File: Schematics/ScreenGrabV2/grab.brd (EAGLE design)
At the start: 48 x 60.4 mm, 48 parts

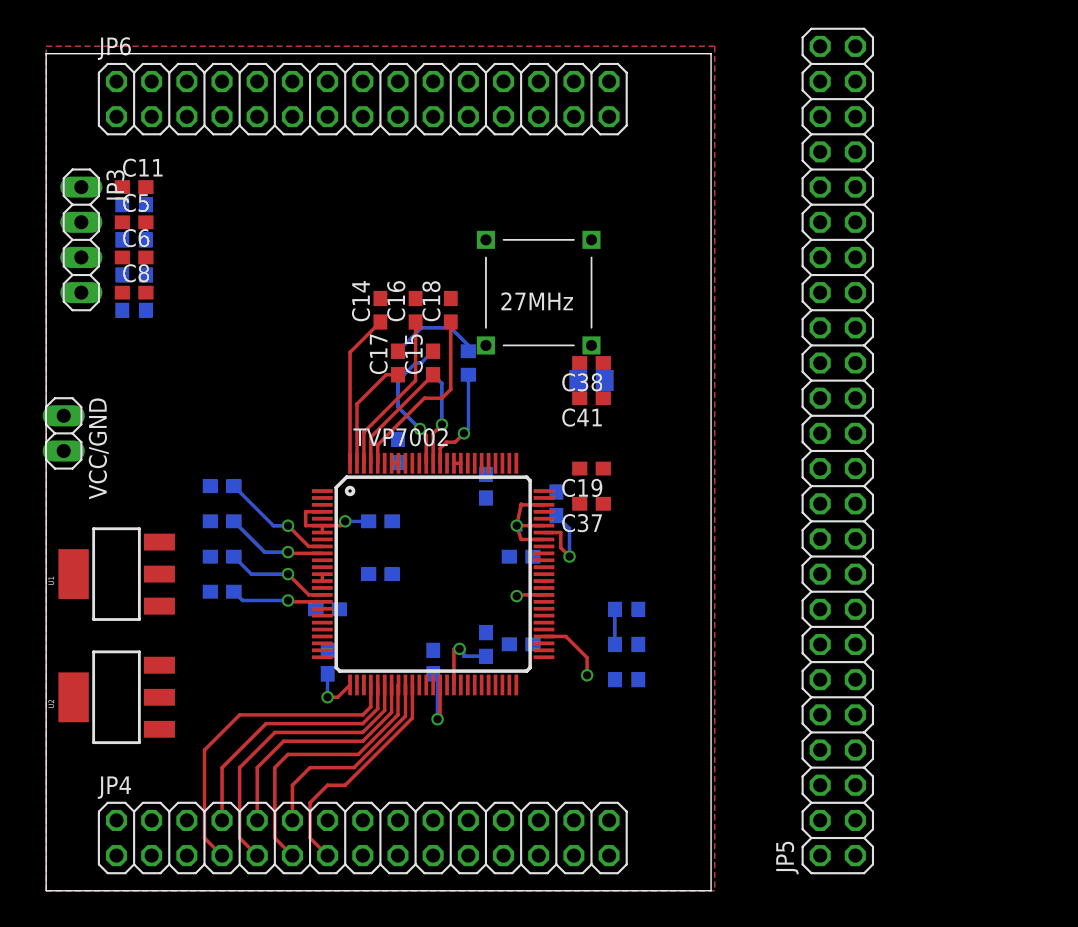
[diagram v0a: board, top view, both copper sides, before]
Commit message: Schematic routed
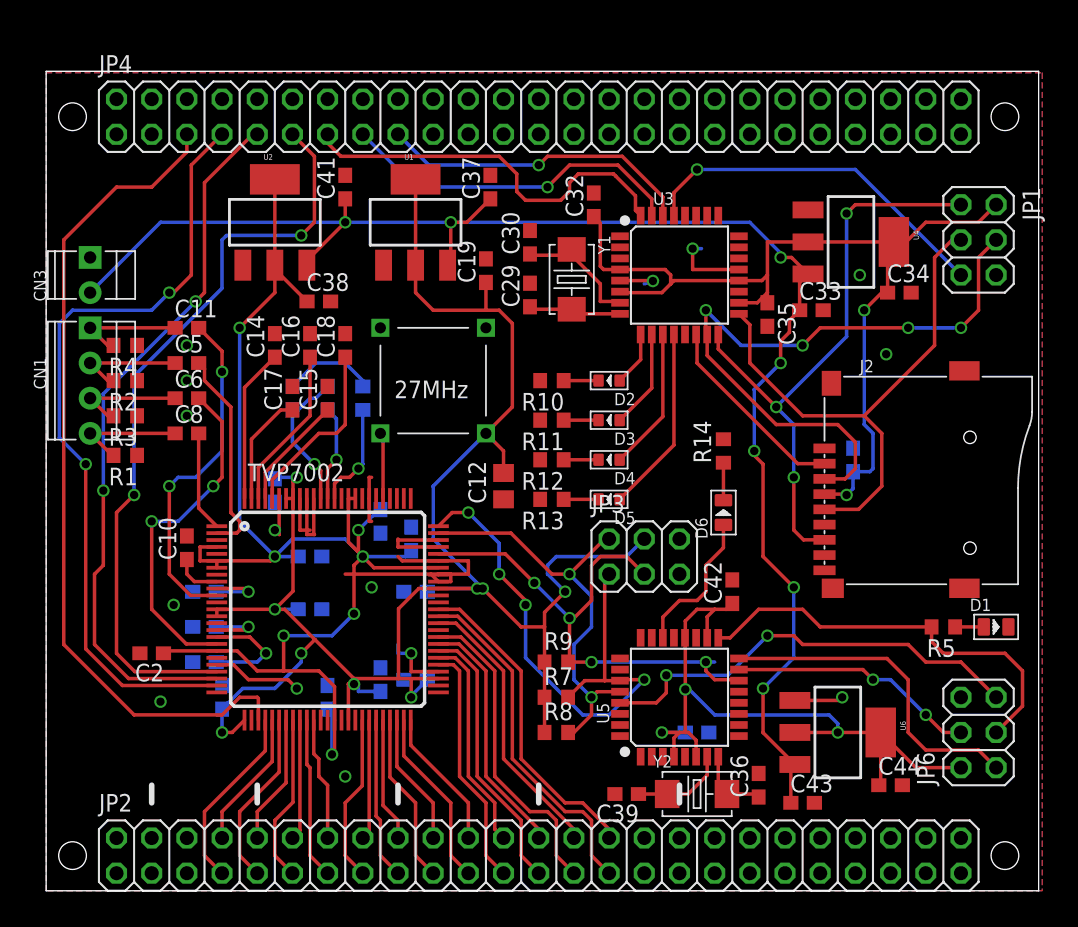
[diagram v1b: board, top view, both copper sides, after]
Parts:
- removed JP5: (no value), pinhead:2X24
- removed VCC/GND: (no value), pinhead:1X02
- added C29, C30, C31, C32, C33, C34, C35, C36, C39, C42, C43, C44, C45: (no value), resistor:C0603
- added CN1: 4p-2.54-h8.5, Seeed-OPL-Connector:H4-2.54-8.52X6.3MM
- added CN3: 2p-2.54-h8.5, Seeed-OPL-Connector:H2-2.54-3.44X6.3MM
- added D1, D6: CLEAR-BLUE-0805, Seeed-OPL-Diode:LED-0805
- added D2, D3, D4, D5: BLUE-0603, Seeed-OPL-Diode:LED-0603
- added J2: MICROSD-9P, Seeed-OPL-Connector:MICRO-SD9+4P-SMD-16.1X14.5X1.85MM
- added JP1: (no value), pinhead:2X03
- added JP2: (no value), pinhead:2X25
- added R10, R11, R12, R13, R14, R5: (no value), resistor:R0603
- added U3, U5: ATMEGA328P-AU-TQFP32, Seeed-OPL-ic:TQFP32-0.8-7X7MM
- added U4, U6: (no value), SparkFun-PowerIC:SOT223
- added Y1, Y2: 16MHZ, Seeed-OPL-crystal-osctllator:X2-SMD-5.0X3.2X1.3MM
- JP3: device pinhead:1X04 -> pinhead:2X03
- JP4: device pinhead:2X15 -> pinhead:2X25
- JP6: device pinhead:2X15 -> pinhead:2X03
- moved JP6 63.8 mm to (67.3, 11.4), turned to 90 degrees
- moved JP4 53.6 mm to (35.6, 55.9)
- moved JP3 46.6 mm to (43.2, 24.1), turned to 0 degrees
- moved U2 36.1 mm to (16.5, 48.3), turned to 0 degrees
- moved U1 33.3 mm to (26.7, 48.3), turned to 0 degrees
- moved C37 24.0 mm to (32.1, 50.8), turned to 90 degrees
- moved C41 23.4 mm to (21.6, 50.8), turned to 90 degrees
- moved C38 20.2 mm to (19.7, 42.5), turned to 0 degrees
- moved C19 16.2 mm to (31.8, 44.8), turned to 90 degrees
- moved C2 13.1 mm to (7.62, 17.1), flipped to the top, turned to 180 degrees
- moved C11 10.9 mm to (10.2, 40.6)
- moved C5 10.9 mm to (10.2, 38.1)
- moved C6 10.9 mm to (10.2, 35.6)
- moved C8 10.9 mm to (10.2, 33.0)
- moved C26 10.8 mm to (26.4, 25.4)
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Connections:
- new net C_MISO: JP6.1, U5.16
- new net C_MOSI: JP6.4, U5.15
- new net C_RST: JP6.5, U5.29
- new net C_SCK: JP6.3, R5.2, U5.17
- new net C_VCC: C42.1, C44.1, C45.1, JP6.2, U5.18, U5.20, U5.4, U5.6, U6.2, U6.4
- new net N$10: C30.1, U3.7, Y1.1
- new net N$11: C29.1, U3.8, Y1.2
- new net N$12: D2.-, R10.1
- new net N$13: D3.-, R11.1
- new net N$14: D4.-, R12.1
- new net N$15: D5.-, R13.1
- new net N$16: D6.+, U5.22
- new net N$17: D6.-, R14.1
- new net N$2: J2.2, U3.14
- new net N$3: D2.+, U3.9
- new net N$4: C39.1, U5.7, Y2.1
- new net N$5: C36.1, U5.8, Y2.2
- new net N$6: D3.+, U3.10
- new net N$7: D4.+, U3.11
- new net N$8: D1.+, R5.1
- new net N$9: D5.+, U3.12
- new net UNUSED1: JP4.17, U3.30
- new net UNUSED2: JP4.15, U3.31
- new net UNUSED3: JP4.13, U3.32
- new net W_MISO: J2.7, JP1.1, U3.16
- new net W_MOSI: J2.3, JP1.4, U3.15
- new net W_RST: JP1.5, U3.29
- new net W_SCK: J2.5, JP1.3, U3.17
- new net W_VCC: C31.1, C32.1, C34.1, C35.1, J2.4, JP1.2, U3.18, U3.20, U3.4, U3.6, U4.2, U4.4
- net +3.3V: now also JP3.4
- net +5V: now also C33.1, C43.1, CN3.2, U4.3, U6.3; no longer VCC/GND.2
- net B0: now also JP2.14; no longer JP4.14
- net B1: now also JP2.13; no longer JP4.13
- net B2: now also JP2.12; no longer JP4.12
- net B3: now also JP2.11; no longer JP4.11
- net B4: now also JP2.10; no longer JP4.10
- net B5: now also JP2.9; no longer JP4.9
- net B6: now also JP2.8; no longer JP4.8
- net B7: now also JP2.7; no longer JP4.7
- net BIN: now also CN1.3; no longer JP3.3
- net CSYNCIN: now also CN1.4; no longer JP3.4
- net FIDOUT: now also JP4.11; no longer JP6.14
- net G0: now also JP2.22; no longer JP4.22
- net G1: now also JP2.21; no longer JP4.21
- net G2: now also JP2.20; no longer JP4.20
- net G3: now also JP2.19; no longer JP4.19
- net G4: now also JP2.18; no longer JP4.18
- net G5: now also JP2.17; no longer JP4.17
- net G6: now also JP2.16; no longer JP4.16
- net G7: now also JP2.15; no longer JP4.15
- net GIN: now also CN1.2; no longer JP3.2
- net GND: now also C29.2, C30.2, C31.2, C32.2, C33.2, C34.2, C35.2, C36.2, C39.2, C42.2, C43.2, C44.2, C45.2, CN3.1, D1.-, J2.6, J2.G1, J2.G2, J2.G3, J2.G4, JP1.6, JP2.2, JP2.4, JP3.5, JP3.6, JP6.6, R10.2, R11.2, R13.2, R14.2, U3.21, U3.3, U3.5, U4.1, U5.21, U5.3, U5.5, U6.1; no longer JP4.2, JP4.4, VCC/GND.1
- net HSOUT: now also JP4.7; no longer JP6.10
- net N$1: now also JP2.1; no longer JP4.1
- net PCLK: now also JP4.5; no longer JP6.8
- net R0: now also JP2.30; no longer JP4.30
- net R1: now also JP2.29; no longer JP4.29
- net R2: now also JP2.28; no longer JP4.28
- net R3: now also JP2.27; no longer JP4.27
- net R4: now also JP2.26; no longer JP4.26
- net R5: now also JP2.25; no longer JP4.25
- net R6: now also JP2.24; no longer JP4.24
- net R7: now also JP2.23; no longer JP4.23
- net RESET: now also JP3.3, U5.14
- net RIN: now also CN1.1; no longer JP3.1
- net SCL: now also JP3.2, U5.28
- net SDA: now also JP3.1, U5.27
- net VSOUT: now also JP4.9; no longer JP6.12
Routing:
- net +3.3V: track 12.7 -> 141.0 mm, vias 2 -> 9
- net +5V: track 0.32 -> 111.4 mm, vias 0 -> 7
- net +1.8V: track 20.4 -> 103.1 mm, vias 3 -> 7
- net W_VCC: track 0.00 -> 68.6 mm, vias 0 -> 2
- net PCLK: track 0.00 -> 60.3 mm
- net HSOUT: track 0.00 -> 56.9 mm, vias 0 -> 2
- net FIDOUT: track 0.00 -> 55.0 mm, vias 0 -> 2
- net VSOUT: track 0.00 -> 51.7 mm, vias 0 -> 2
- net C_VCC: track 0.00 -> 51.3 mm, vias 0 -> 3
- net W_MOSI: track 0.00 -> 48.4 mm, vias 0 -> 4
- net GND: track 16.0 -> 63.7 mm, vias 3 -> 15
- net W_MISO: track 0.00 -> 43.5 mm, vias 0 -> 3
- net W_SCK: track 0.00 -> 40.1 mm
- net SDA: track 0.00 -> 39.9 mm, vias 0 -> 4
- net RESET: track 0.00 -> 37.7 mm, vias 0 -> 4
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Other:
- board size 48 x 60.4 mm -> 71.7 x 59.2 mm

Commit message: Schematic update
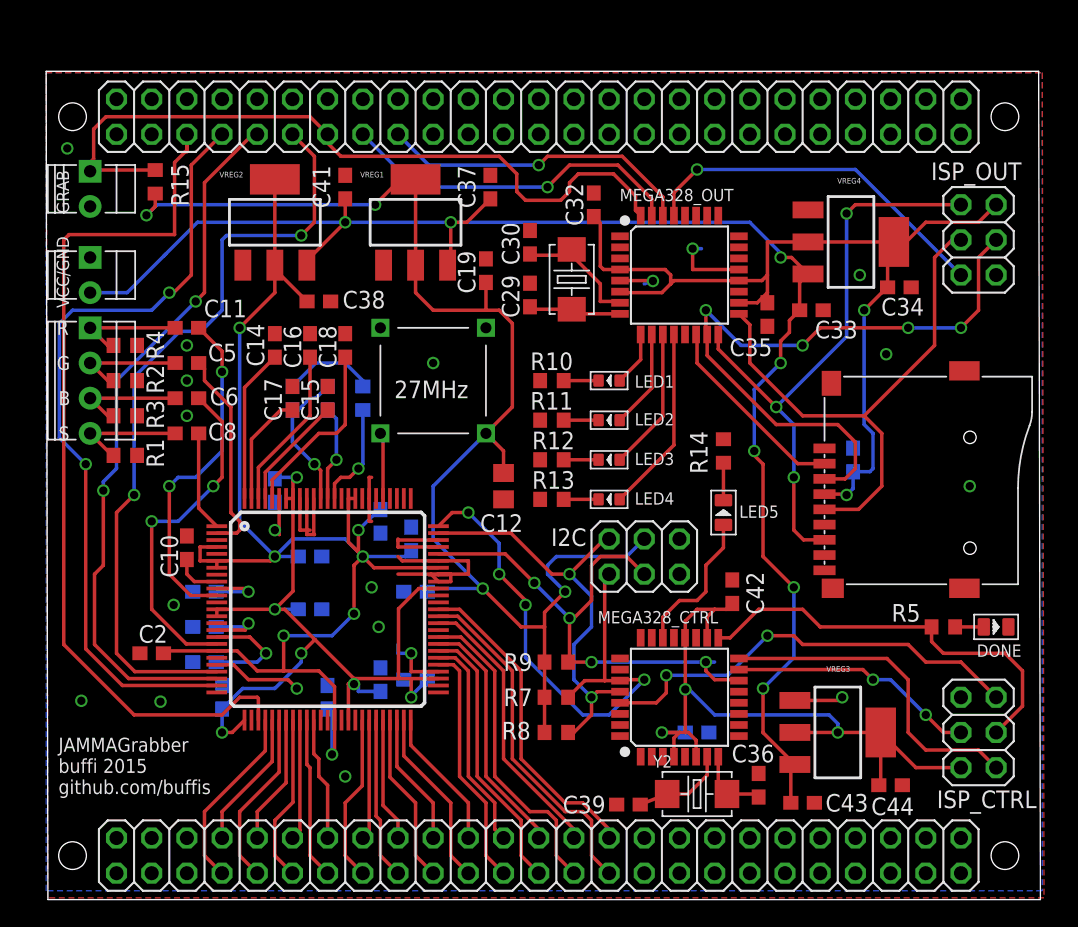
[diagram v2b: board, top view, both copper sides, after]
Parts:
- added GRAB: 2p-2.54-h8.5, Seeed-OPL-Connector:H2-2.54-3.44X6.3MM
- added R15: 10K, resistor:R0603
- VREG1, VREG3, VREG4: value (none) -> 3.3V
- VREG2: value (none) -> 1.8V
- moved C39 0.77 mm to (42.0, 6.22)
- moved C34 0.38 mm to (61.6, 43.6)
- renumbered CN3 to VCC/GND, D1 to DONE, D2 to LED1, D3 to LED2, D4 to LED3, D5 to LED4, D6 to LED5, JP1 to ISP_OUT, JP3 to I2C, JP6 to ISP_CTRL, U1 to VREG1, U2 to VREG2, U3 to MEGA328_OUT, U4 to VREG4, U5 to MEGA328_CTRL, U6 to VREG3
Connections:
- removed net UNUSED3: JP4.13, MEGA328_OUT.32
- new net CAPTURE: GRAB.1, JP4.13, MEGA328_OUT.32, R15.2
- net +3.3V: now also R15.1
- net GND: now also GRAB.2
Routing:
- net CAPTURE: track 0.00 -> 53.7 mm
- net UNUSED3: track 28.7 -> 0.00 mm
- net +3.3V: track 141.0 -> 160.5 mm, vias 9 -> 10
- net PCLK: track 60.3 -> 64.5 mm
- net GND: track 63.7 -> 59.9 mm, vias 15 -> 20
- net FIDOUT: track 55.0 -> 55.9 mm
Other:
- board size 71.7 x 59.2 mm -> 71.8 x 59.8 mm
- board text added: "B"
- board text added: "G"
- board text added: "JAMMAGrabber buffi 2015 github.com/buffis"
- board text added: "R"
- board text added: "S"
